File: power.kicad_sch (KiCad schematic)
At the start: 14 parts, among them U3 TLV71333PDQN

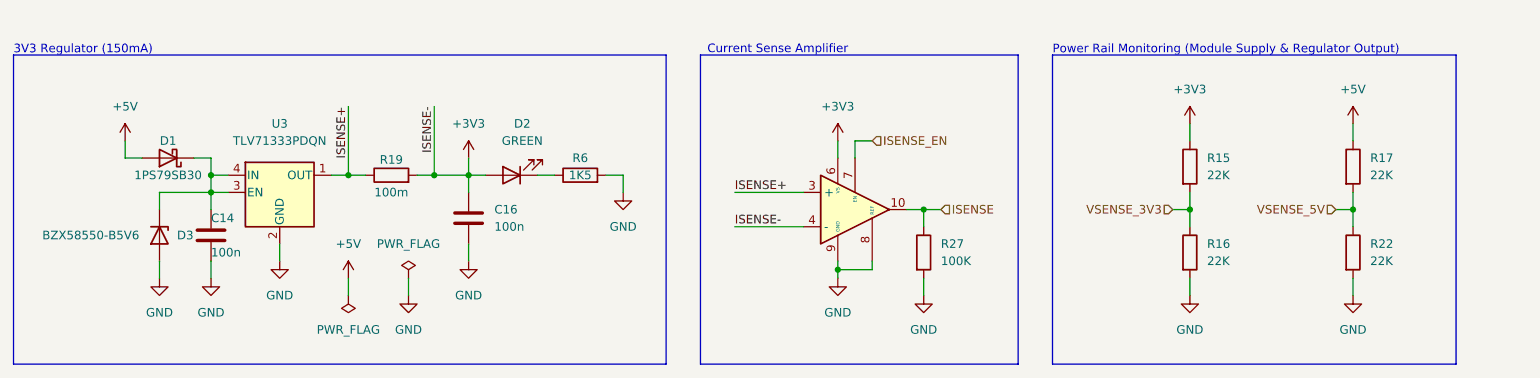
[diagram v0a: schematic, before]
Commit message: schematic: cleanup
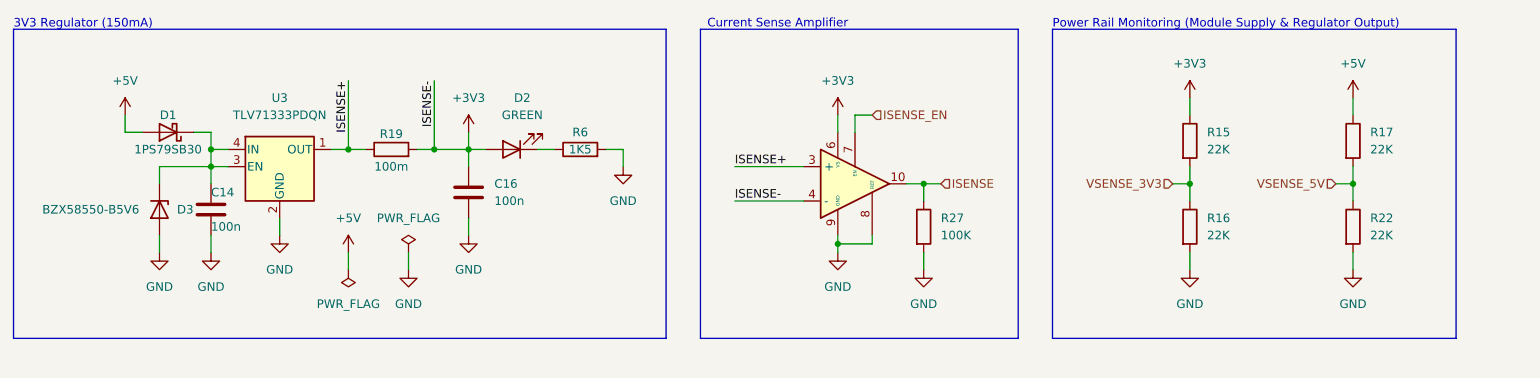
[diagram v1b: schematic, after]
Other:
- moved on the sheet: C14, C16, D1, D2, D3, R15, R16, R17, R19, R22, R27, R6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

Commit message: schematic: footprint assignment
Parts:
- R19: footprint (none) -> Resistor_SMD:R_0603_1608Metric
- R27: footprint (none) -> Resistor_SMD:R_0201_0603Metric
- U9: footprint (none) -> Package_DFN_QFN:Texas_RSW0010A_UQFN-10_1.4x1.8mm_P0.4mm
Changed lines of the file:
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@@
 			)
 		)
-		(property "Footprint" ""
+		(property "Footprint" "Package_DFN_QFN:Texas_RSW0010A_UQFN-10_1.4x1.8mm_P0.4mm"
 			(at 139.7 43.18 0)
 			(effects
@@
 		(pin "7"
 		)
-		(pin "4"
-		)
 		(pin "6"
 		)
@@
 			)
 		)
-		(property "Footprint" ""
+		(property "Footprint" "Resistor_SMD:R_0201_0603Metric"
 			(at 149.352 49.53 90)
 			(effects
@@
 			)
 		)
-		(property "Footprint" ""
+		(property "Footprint" "Resistor_SMD:R_0603_1608Metric"
 			(at 72.39 39.878 90)
 			(effects
